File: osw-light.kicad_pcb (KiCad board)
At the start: 4 copper layers, 36.1 x 36.1 mm, 55 parts, among them J1 Conn_01x02, Q1 2N7002, SW1 SW_Push, SW2 SW_Push, SW4 SW_Push, SW5 SW_Push, U1 DS3231MZ, U10 XC6209, U11 MCP73831T-2ACI_OT, U13 XC6209, U2 BMA400, U4 GC9A01_IPS_display, U5 USB-OTG, U6 CH340E, U7 ttgo-32-micro, U9 TPS2115A

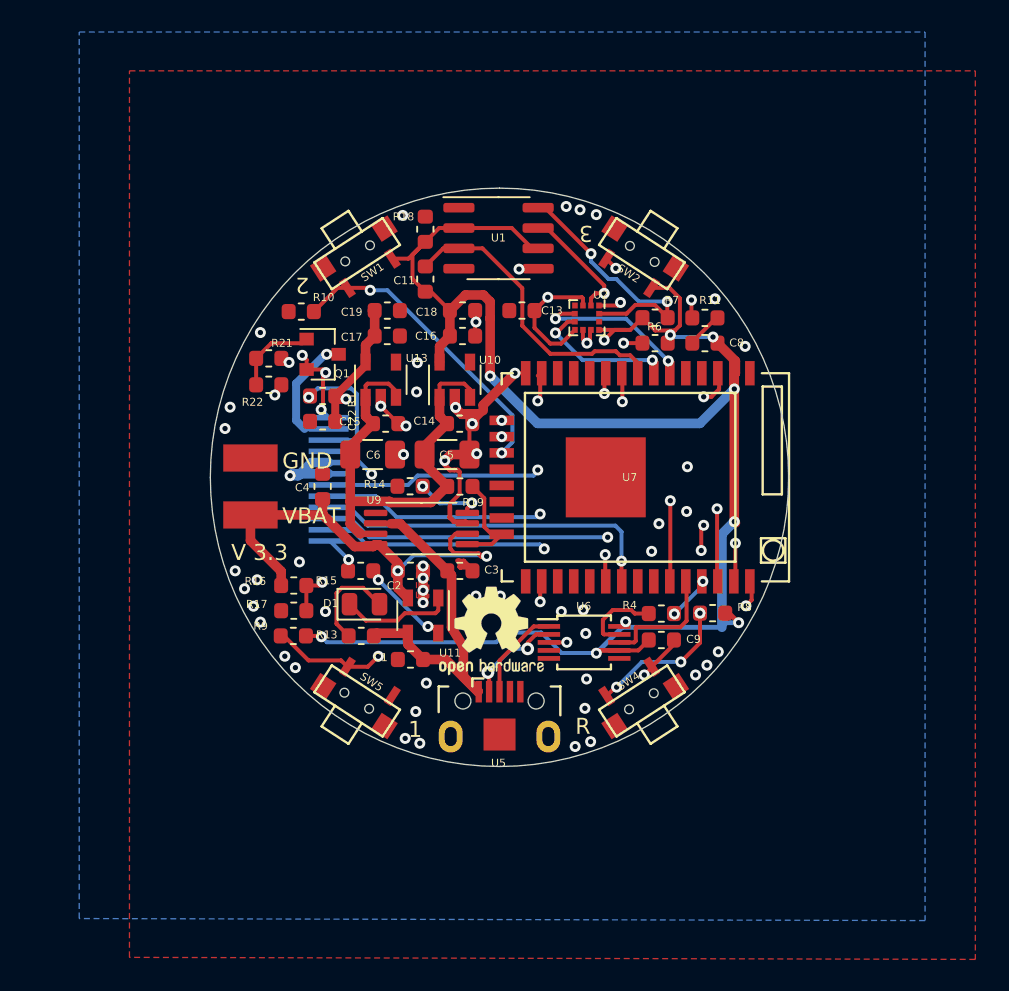
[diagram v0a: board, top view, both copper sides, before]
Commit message: Added type c
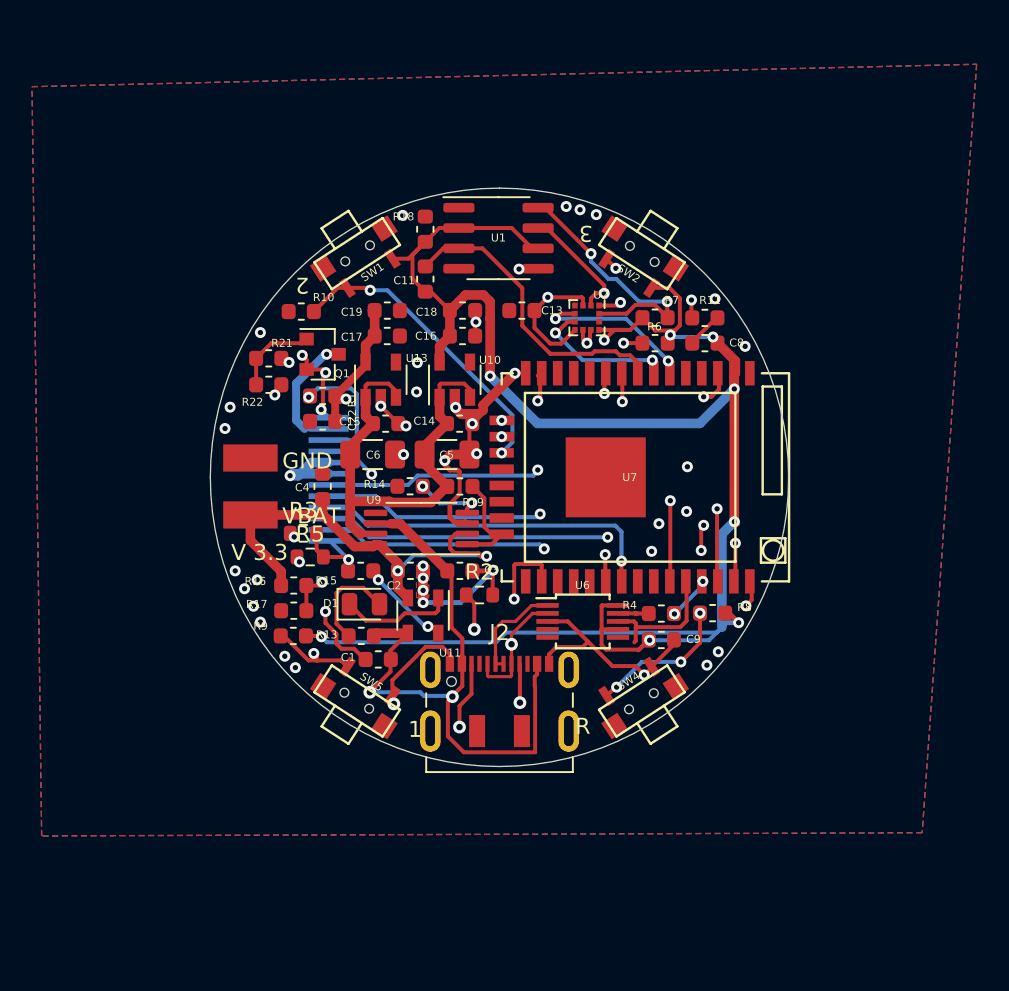
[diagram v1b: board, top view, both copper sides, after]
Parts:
- removed the REF** at (75.7, 111.2)
- removed U5: USB-OTG, open-Smartwatch:USBmicro-B
- added J2: USB_C_Receptacle_USB2.0_14P, Connector_USB:USB_C_Receptacle_JAE_DX07S016JA1R1500, F.Cu at (76.2, 116.3)
- added R2: 1M, Resistor_SMD:R_0603_1608Metric, F.Cu at (75.0, 109.0)
- added R3: 5.11k, Resistor_SMD:R_0603_1608Metric, F.Cu at (64.0, 105.1)
- added R5: 5.11k, Resistor_SMD:R_0603_1608Metric, F.Cu at (64.4, 106.6)
- moved C1 2.01 mm to (68.6, 113.0)
- moved U6 1.32 mm to (81.4, 110.6)
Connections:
- U1 pad 1: Net-(U1-Pad1) -> unconnected-(U1-32KHZ-Pad1)
- U1 pad 4: Net-(U1-Pad4) -> unconnected-(U1-~{RST}-Pad4)
- U10 pad 4: Net-(U10-Pad4) -> unconnected-(U10-NC-Pad4)
- U13 pad 4: Net-(U13-Pad4) -> unconnected-(U13-NC-Pad4)
- U2 pad 11: Net-(U2-Pad11) -> unconnected-(U2-NC-Pad11)
- U2 pad 4: Net-(U2-Pad4) -> unconnected-(U2-NC-Pad4)
- U6 pad 4: Net-(U6-Pad4) -> unconnected-(U6-~{RTS}-Pad4)
- U6 pad 5: Net-(U6-Pad5) -> unconnected-(U6-~{CTS}-Pad5)
- U6 pad 6: Net-(U6-Pad6) -> unconnected-(U6-TNOW-Pad6)
- U7 pad 11: Net-(U7-Pad11) -> unconnected-(U7-IO26-Pad11)
- U7 pad 12: Net-(U7-Pad12) -> unconnected-(U7-IO27-Pad12)
- U7 pad 13: Net-(U7-Pad13) -> unconnected-(U7-IO14-Pad13)
- U7 pad 19: Net-(U7-Pad19) -> unconnected-(U7-SD2-Pad19)
- U7 pad 20: Net-(U7-Pad20) -> unconnected-(U7-CLK-Pad20)
- U7 pad 21: Net-(U7-Pad21) -> unconnected-(U7-SD3-Pad21)
- U7 pad 22: Net-(U7-Pad22) -> unconnected-(U7-SD1-Pad22)
- U7 pad 24: Net-(U7-Pad24) -> unconnected-(U7-IO02-Pad24)
- U7 pad 26: Net-(U7-Pad26) -> unconnected-(U7-IO04-Pad26)
- U7 pad 27: Net-(U7-Pad27) -> unconnected-(U7-CS-Pad27)
- U7 pad 28: Net-(U7-Pad28) -> unconnected-(U7-SD0-Pad28)
- U7 pad 31: Net-(U7-Pad31) -> unconnected-(U7-IO19-Pad31)
- U7 pad 32: Net-(U7-Pad32) -> unconnected-(U7-NC-Pad32)
- U7 pad 4: Net-(U7-Pad4) -> unconnected-(U7-VP-Pad4)
- U7 pad 5: Net-(U7-Pad5) -> unconnected-(U7-VN-Pad5)
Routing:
- net GND: track 64.5 -> 94.3 mm, vias 65 -> 51
- net Net-(J2-CC2): track 0.00 -> 25.8 mm, vias 0 -> 2
- net Net-(J2-SHIELD): track 0.00 -> 25.7 mm, vias 0 -> 1
- net Net-(J2-CC1): track 0.00 -> 19.7 mm, vias 0 -> 2
- net /VBUS: track 22.4 -> 41.0 mm, vias 0 -> 2
- net +3V3: track 126.3 -> 134.3 mm, vias 11 -> 10
- net /FLASH: track 20.0 -> 24.5 mm
- net Net-(U6-RXD): track 5.10 -> 2.08 mm
- net /D_N: track 6.25 -> 7.80 mm, vias 2 -> 1
- net /D_P: track 5.91 -> 6.70 mm
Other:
- net class Default removed
